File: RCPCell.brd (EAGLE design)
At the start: 99.8 x 44.5 mm, 18 parts, among them IC1 SIM900, U1 PESDXS4UD

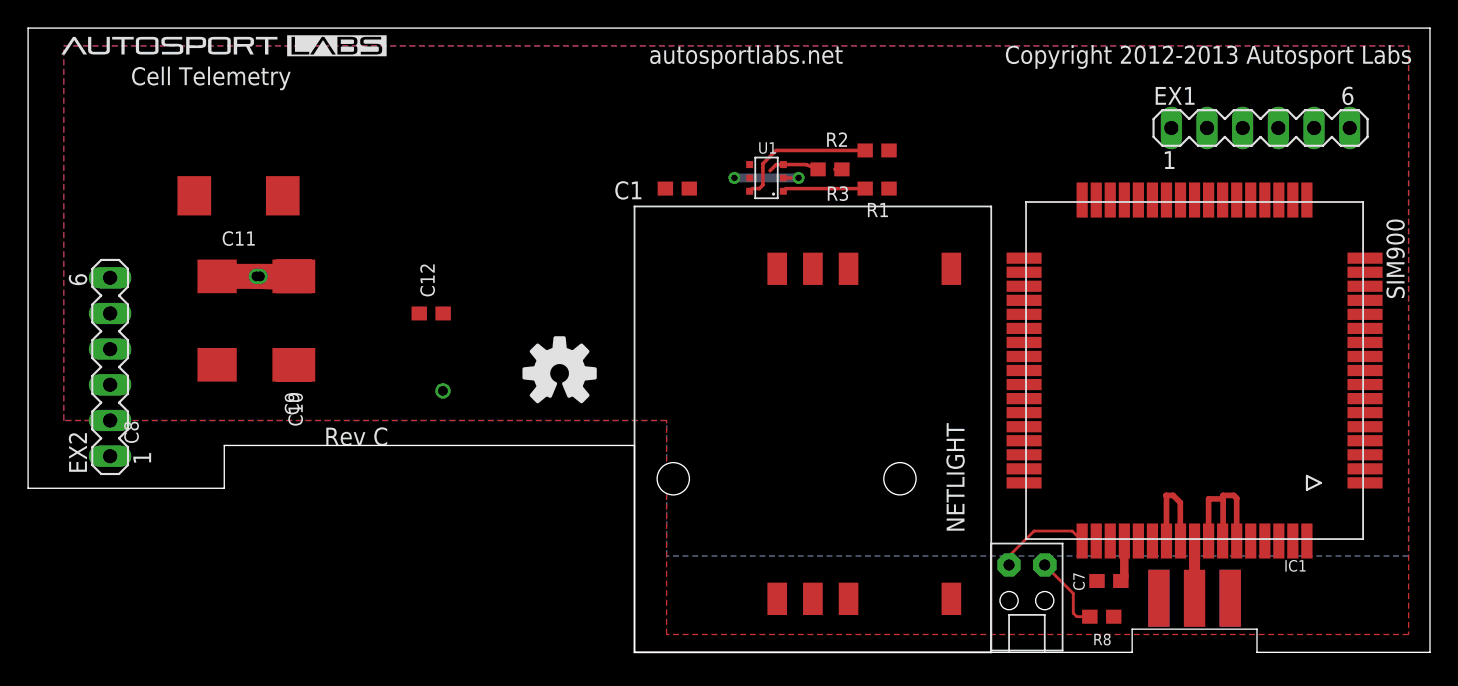
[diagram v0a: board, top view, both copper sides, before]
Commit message: final layout before incorporating power supply section
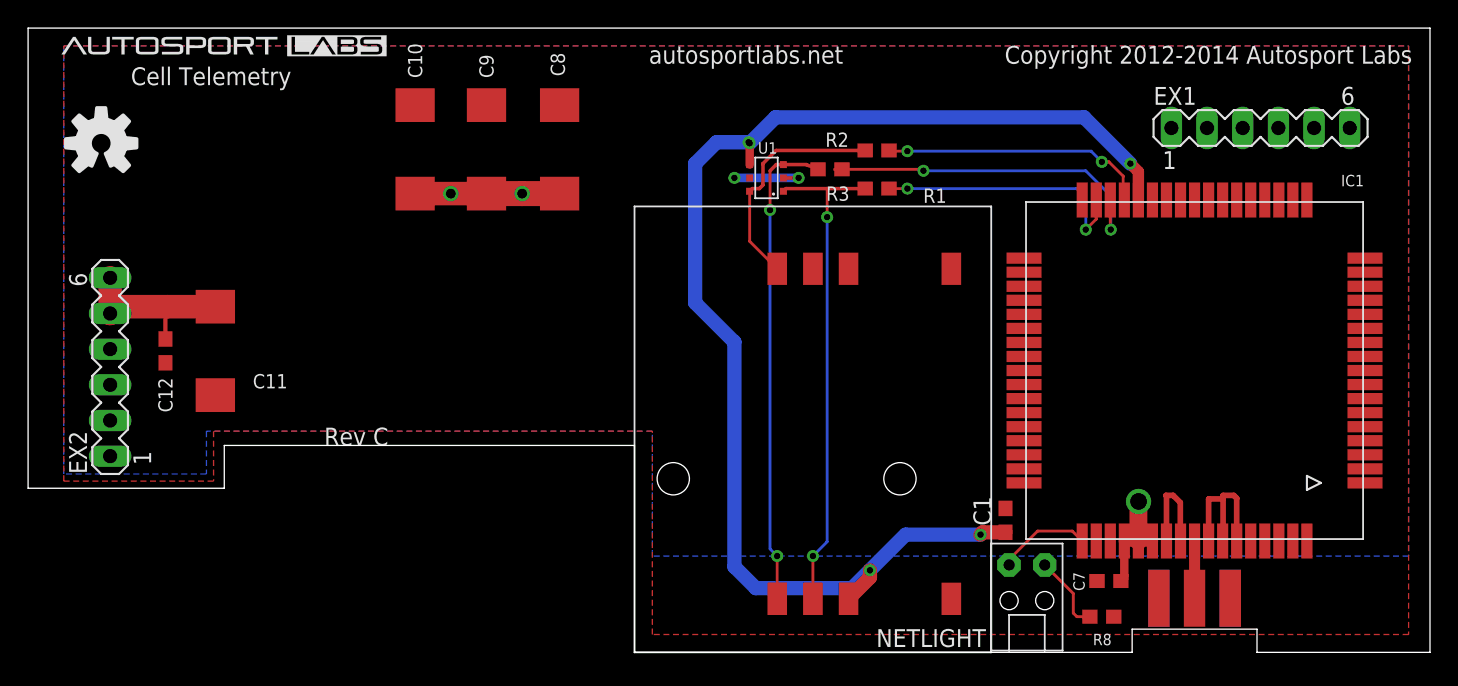
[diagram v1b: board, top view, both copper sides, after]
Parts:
- moved C1 33.2 mm to (69.6, 9.40), turned to 90 degrees
- moved C8 27.3 mm to (37.8, 35.8), turned to 90 degrees
- moved C12 19.1 mm to (9.78, 21.5), turned to 270 degrees
- moved C9 18.4 mm to (32.6, 35.8), turned to 90 degrees
- moved C10 14.9 mm to (27.6, 35.8), turned to 90 degrees
- moved C11 11.2 mm to (13.3, 21.5), turned to 270 degrees
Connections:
- net +5V: no longer C11.+
- net SAFE12V: now also C11.+, C12.1
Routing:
- net SIM_VDD: track 0.00 -> 92.2 mm, vias 0 -> 5
- net SIM_CLK_CARD: track 3.67 -> 34.4 mm, vias 0 -> 2
- net SIM_RST_CARD: track 5.90 -> 35.5 mm, vias 0 -> 2
- net SIM_CLK: track 0.50 -> 25.0 mm, vias 0 -> 2
- net SIM_DATA: track 0.50 -> 19.2 mm, vias 0 -> 2
- net SIM_RST: track 0.52 -> 19.0 mm, vias 0 -> 2
- net SAFE12V: track 0.00 -> 12.6 mm
- net V+: track 11.2 -> 20.6 mm
- net SIM_DATA_CARD: track 10.3 -> 16.7 mm
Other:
- board text added: "Copyright 2012-2014 Autosport Labs"
- board text removed: "Copyright 2012-2013 Autosport Labs"
